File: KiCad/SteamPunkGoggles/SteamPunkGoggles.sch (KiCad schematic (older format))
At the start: 7 parts

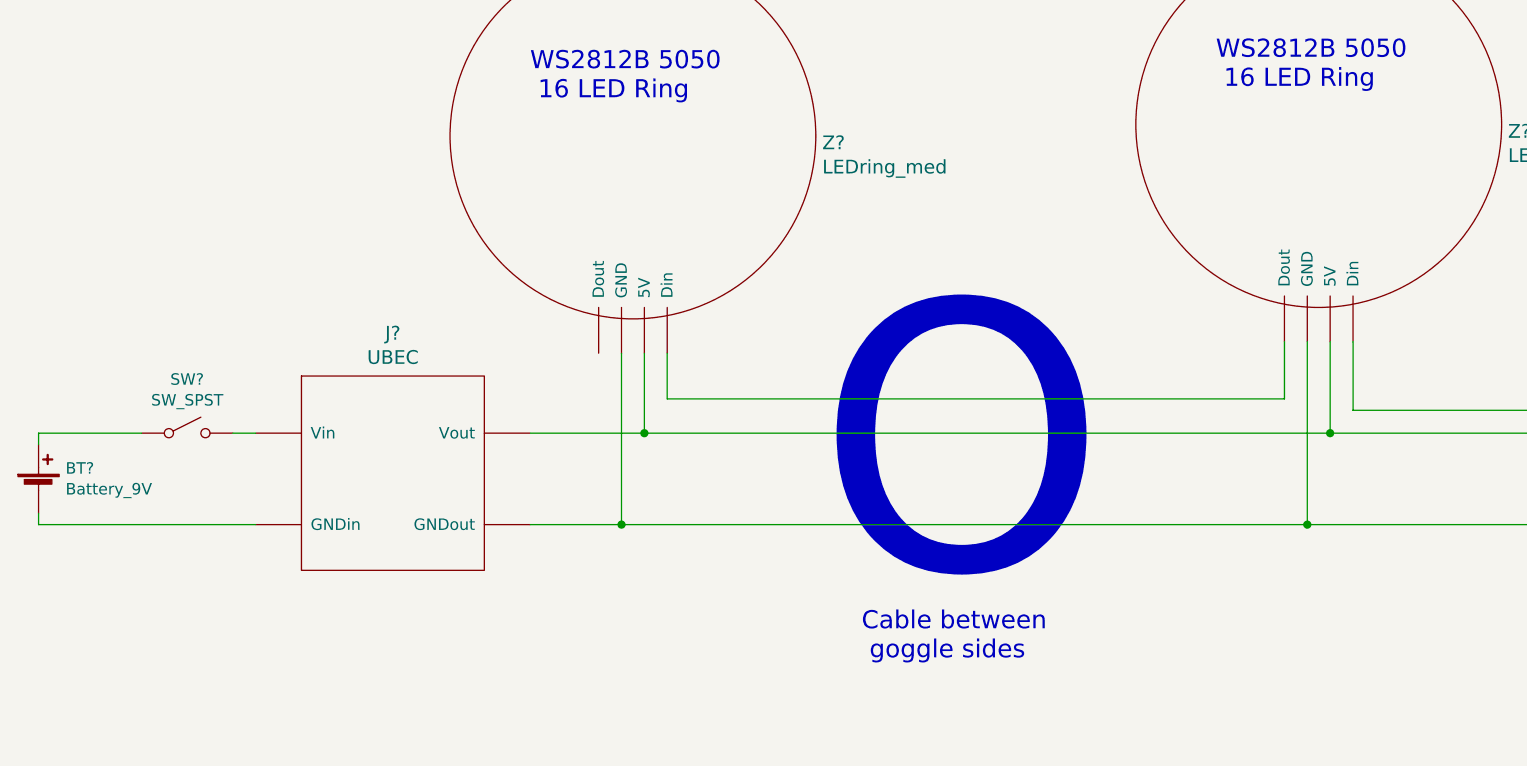
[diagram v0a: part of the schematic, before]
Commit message: annotate schematic
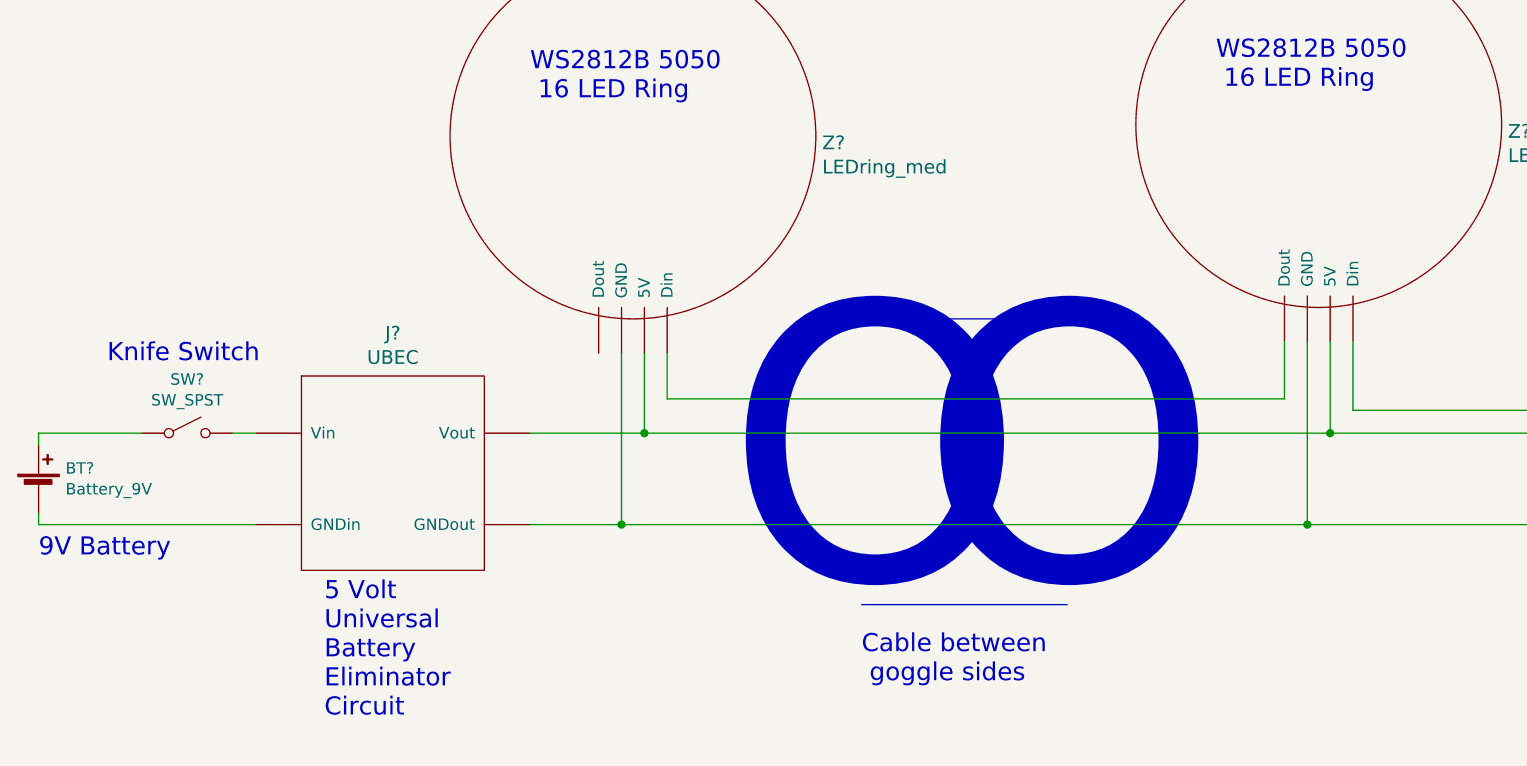
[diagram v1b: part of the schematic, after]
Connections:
- net at A?.~ (VIN): now also Z?.~ (GND)
- net at Z?.~ (GND), Z?.~ (GND): no longer A?.~ (VIN), J?.~ (Vout)
- new net: A?.~ (VIN), J?.~ (Vout), RV?.1, Z?.~ (GND), Z?.~ (GND)
- new net: A?.~ (VIN), J?.~ (Vout), Z?.~ (GND), Z?.~ (GND)
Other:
- note added: "5 Volt\nUniversal\nBattery\nEliminator\nCircuit"
- note added: "9V Battery"
- note added: "Knife Switch"
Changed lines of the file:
@@
 Sheet 1 1
 Title "Steam Punk Goggles from KnowHow187"
-Date "2023-01-27"
+Date "2023-02-03"
 Rev ""
 Comp "MDO"
@@
 	2900 5250 3300 5250
 Connection ~ 3300 5250
-Text Notes 4150 5600 0    1181 ~ 0
-O
-Text Notes 4350 5850 0    79   ~ 0
+Text Notes 4350 5950 0    79   ~ 0
 Cable between\n goggle sides
 Text Notes 1750 1450 0    197  ~ 0
 9V rechargeable battery and UBEC on one side\nArduino Nano and potentiometer on other side
+Wire Bus Line
+	4350 4350 5250 4350
+Text Notes 3750 5650 0    1220 ~ 0
+O
+Text Notes 4600 5650 0    1220 ~ 0
+O
+Wire Bus Line
+	4350 5600 5250 5600
+Text Notes 1050 4550 0    79   ~ 0
+Knife Switch
+Text Notes 2000 6100 0    79   ~ 0
+5 Volt\nUniversal\nBattery\nEliminator\nCircuit
+Text Notes 750  5400 0    79   ~ 0
+9V Battery
 $EndSCHEMATC
